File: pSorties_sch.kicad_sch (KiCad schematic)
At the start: 29 parts, among them K1 G6DN-1A-L DC24, K2 G6DN-1A-L DC24, Q1 2N7002, Q2 2N7002, U3 DRV81545PWPR, U4 ISO6420FDR, U5 TLV709A50DBVR

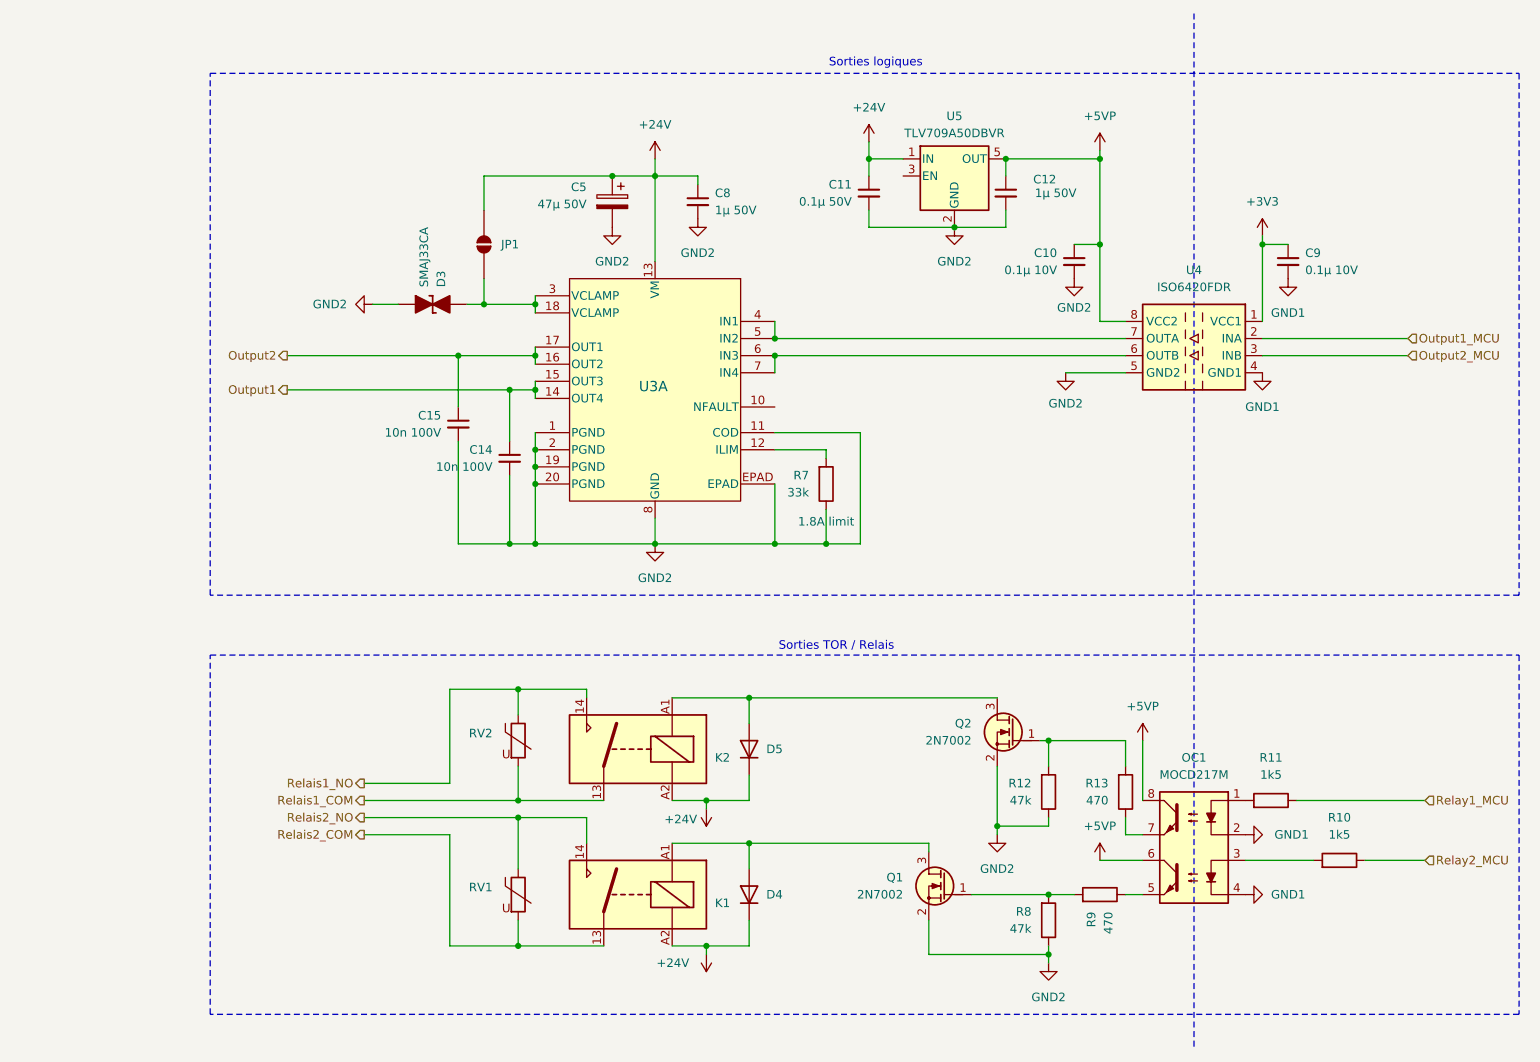
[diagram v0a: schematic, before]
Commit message: avant prod
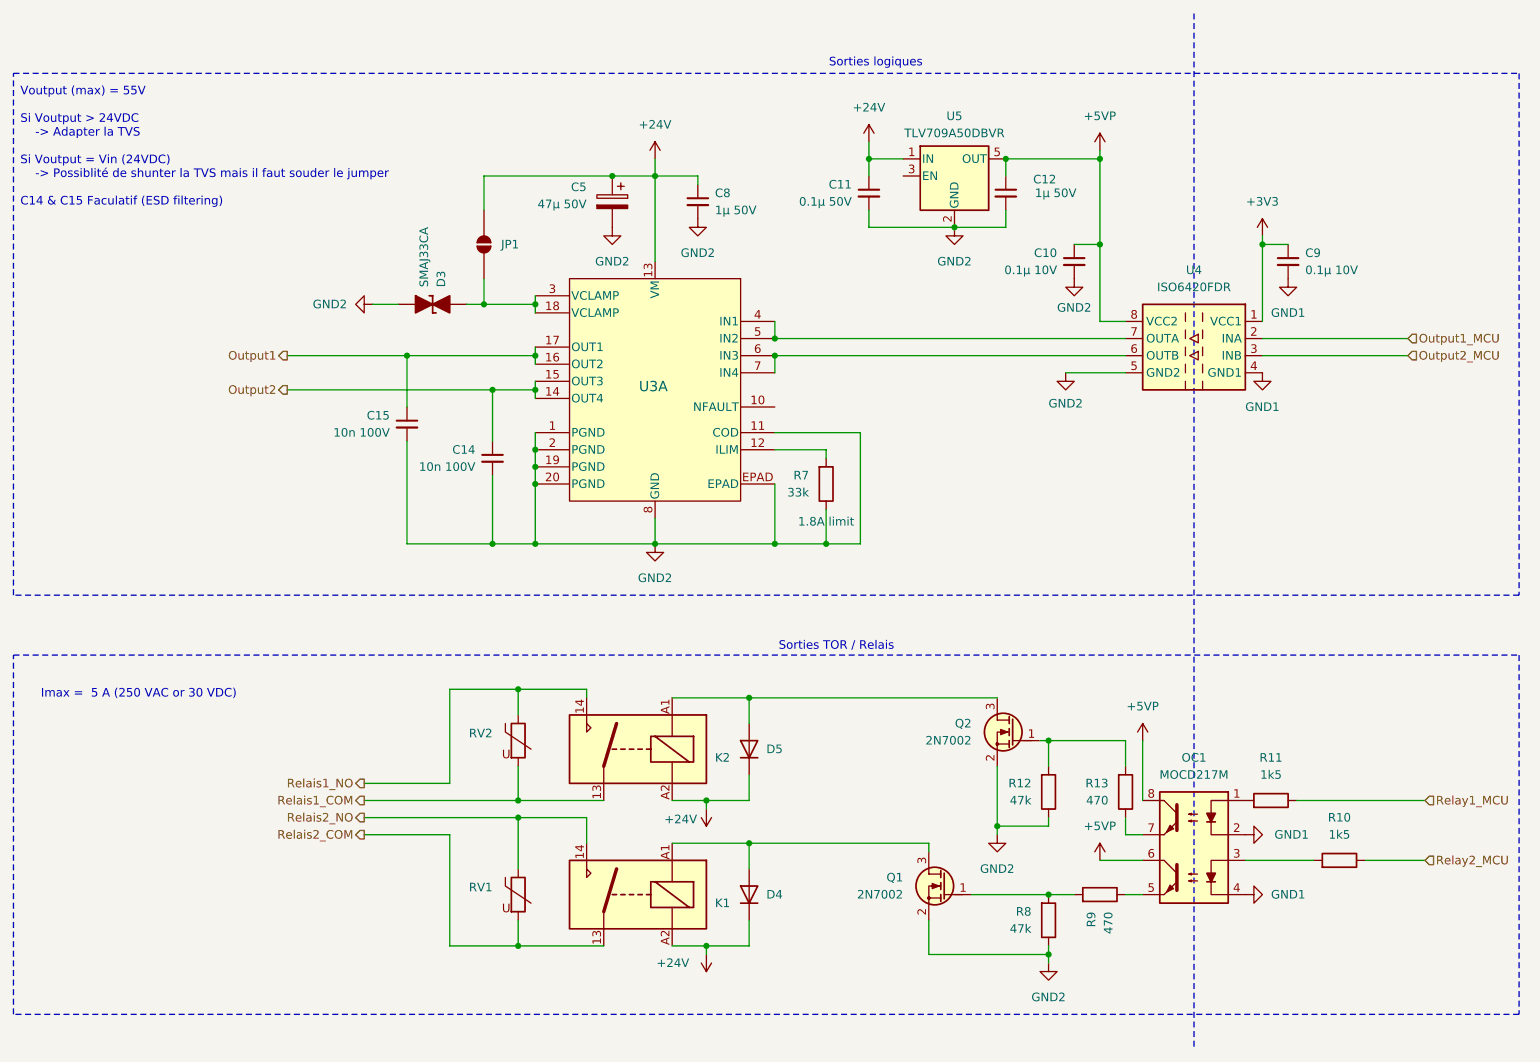
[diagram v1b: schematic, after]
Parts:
- OC1: LCSC Part # (none) -> C258262
- Q1, Q2: LCSC Part # (none) -> C8545
- U3: LCSC Part # (none) -> C53201928
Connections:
- net Output1: now also C15.1, U3.16 (OUT2), U3.17 (OUT1); no longer C14.1, U3.14 (OUT4), U3.15 (OUT3)
- net Output2: now also C14.1, U3.14 (OUT4), U3.15 (OUT3); no longer C15.1, U3.16 (OUT2), U3.17 (OUT1)
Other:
- note added: "Imax = 5 A (250 VAC or 30 VDC)"
- note added: "Voutput (max) = 55V Si Voutput > 24VDC -> Adapter la TVS Si Voutput = Vin (24VDC) -> Possiblité de shunter la TVS mais il faut souder le jumper C14 & C15 Faculatif (ESD filtering)"
- moved on the sheet: C14, C15
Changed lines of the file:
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@@
 	(paper "A4")
 	(rectangle
-		(start 62.23 21.59)
+		(start 33.02 21.59)
 		(end 256.54 99.06)
 		(stroke
@@
 	)
 	(rectangle
-		(start 62.23 107.95)
+		(start 33.02 107.95)
 		(end 256.54 161.29)
 		(stroke
@@
 		)
 	)
+	(text "Voutput (max) = 55V\n\nSi Voutput > 24VDC \n	-> Adapter la TVS\n\nSi Voutput = Vin (24VDC)\n	-> Possiblité de shunter la TVS mais il faut souder le jumper\n\nC14 & C15 Faculatif (ESD filtering)"
+		(exclude_from_sim no)
+		(at 34.036 23.622 0)
+		(effects
+			(font
+				(size 1.27 1.27)
+			)
+			(justify left top)
+		)
+	)
+	(text "Imax =  5 A (250 VAC or 30 VDC)"
+		(exclude_from_sim no)
+		(at 37.084 113.03 0)
+		(effects
+			(font
+				(size 1.27 1.27)
+			)
+			(justify left top)
+		)
+	)
 	(text "Sorties logiques"
 		(exclude_from_sim no)
@@
 	)
 	(junction
-		(at 106.68 68.58)
-		(diameter 0)
-		(color 0 0 0 0)
-	)
-	(junction
 		(at 146.05 63.5)
 		(diameter 0)
@@
 	)
 	(junction
-		(at 99.06 63.5)
+		(at 186.69 152.4)
 		(diameter 0)
 		(color 0 0 0 0)
 	)
 	(junction
-		(at 106.68 91.44)
+		(at 142.24 135.89)
 		(diameter 0)
 		(color 0 0 0 0)
 	)
 	(junction
-		(at 186.69 152.4)
+		(at 104.14 68.58)
 		(diameter 0)
 		(color 0 0 0 0)
 	)
 	(junction
-		(at 142.24 135.89)
+		(at 135.89 151.13)
 		(diameter 0)
 		(color 0 0 0 0)
 	)
 	(junction
-		(at 135.89 151.13)
+		(at 142.24 114.3)
 		(diameter 0)
 		(color 0 0 0 0)
 	)
 	(junction
-		(at 142.24 114.3)
+		(at 146.05 91.44)
 		(diameter 0)
 		(color 0 0 0 0)
 	)
 	(junction
-		(at 146.05 91.44)
+		(at 91.44 63.5)
 		(diameter 0)
 		(color 0 0 0 0)
@@
 	)
 	(junction
+		(at 104.14 91.44)
+		(diameter 0)
+		(color 0 0 0 0)
+	)
+	(junction
 		(at 153.67 91.44)
 		(diameter 0)
@@
 	(wire
 		(pts
-			(xy 106.68 91.44) (xy 110.49 91.44)
-		)
-		(stroke
-			(width 0)
-			(type default)
-		)
-	)
-	(wire
-		(pts
 			(xy 198.12 66.04) (xy 189.23 66.04)
 		)
@@
 	(wire
 		(pts
-			(xy 106.68 81.28) (xy 106.68 91.44)
+			(xy 104.14 81.28) (xy 104.14 91.44)
 		)
 		(stroke
@@
 	(wire
 		(pts
-			(xy 73.66 63.5) (xy 99.06 63.5)
+			(xy 73.66 63.5) (xy 91.44 63.5)
 		)
 		(stroke
@@
 	(wire
 		(pts
+			(xy 104.14 68.58) (xy 110.49 68.58)
+		)
+		(stroke
+			(width 0)
+			(type default)
+		)
+	)
+	(wire
+		(pts
 			(xy 142.24 125.73) (xy 142.24 129.54)
 		)
@@
 	(wire
 		(pts
-			(xy 99.06 63.5) (xy 99.06 71.12)
+			(xy 91.44 63.5) (xy 91.44 71.12)
 		)
 		(stroke
@@
 	(wire
 		(pts
-			(xy 106.68 68.58) (xy 106.68 76.2)
+			(xy 104.14 68.58) (xy 104.14 76.2)
 		)
 		(stroke
@@
 	(wire
 		(pts
-			(xy 99.06 91.44) (xy 106.68 91.44)
+			(xy 91.44 91.44) (xy 104.14 91.44)
 		)
 		(stroke
@@
 	(wire
 		(pts
-			(xy 73.66 68.58) (xy 106.68 68.58)
+			(xy 73.66 68.58) (xy 104.14 68.58)
 		)
 		(stroke
@@
 	(wire
 		(pts
+			(xy 91.44 63.5) (xy 110.49 63.5)
+		)
+		(stroke
+			(width 0)
+			(type default)
+		)
+	)
+	(wire
+		(pts
 			(xy 85.09 132.08) (xy 107.95 132.08)
 		)
@@
 	(wire
 		(pts
+			(xy 104.14 91.44) (xy 110.49 91.44)
+		)
+		(stroke
+			(width 0)
+			(type default)
+		)
+	)
+	(wire
+		(pts
 			(xy 130.81 114.3) (xy 142.24 114.3)
 		)
@@
 	(wire
 		(pts
-			(xy 99.06 76.2) (xy 99.06 91.44)
+			(xy 91.44 76.2) (xy 91.44 91.44)
 		)
 		(stroke
@@
 	(wire
 		(pts
-			(xy 106.68 68.58) (xy 110.49 68.58)
-		)
-		(stroke
-			(width 0)
-			(type default)
-		)
-	)
-	(wire
-		(pts
 			(xy 218.44 45.72) (xy 218.44 46.99)
 		)
@@
 	(wire
 		(pts
-			(xy 99.06 63.5) (xy 110.49 63.5)
-		)
-		(stroke
-			(width 0)
-			(type default)
-		)
-	)
-	(wire
-		(pts
 			(xy 194.31 46.99) (xy 194.31 58.42)
 		)
@@
 		)
 	)
-	(hierarchical_label "Output1"
+	(hierarchical_label "Output2"
 		(shape output)
 		(at 73.66 68.58 180)
@@
 		)
 	)
-	(hierarchical_label "Output2"
+	(hierarchical_label "Output1"
 		(shape output)
 		(at 73.66 63.5 180)
@@
 			)
 		)
+		(property "LCSC Part #" "C8545"
+			(at 171.45 142.24 0)
+			(hide yes)
+			(show_name no)
+			(do_not_autoplace no)
+			(effects
+				(font
+					(size 1.27 1.27)
+				)
+			)
+		)
 		(pin "3"
 		)
@@
 			)
 		)
+		(property "LCSC Part #" "C258262"
+			(at 208.28 132.08 0)
+			(hide yes)
+			(show_name no)
+			(do_not_autoplace no)
+			(effects
+				(font
+					(size 1.27 1.27)
+				)
+			)
+		)
 		(pin "1"
 		)
@@
 	(symbol
 		(lib_id "Device:C_Small")
-		(at 99.06 73.66 0)
+		(at 91.44 73.66 0)
 		(mirror y)
 		(unit 1)
@@
 		(dnp no)
 		(property "Reference" "C15"
-			(at 96.52 72.3962 0)
+			(at 88.9 72.3962 0)
 			(show_name no)
 			(do_not_autoplace no)
@@
 		)
 		(property "Value" "10n 100V"
-			(at 96.52 74.9362 0)
+			(at 88.9 74.9362 0)
 			(show_name no)
 			(do_not_autoplace no)
@@
 		)
 		(property "Footprint" "Capacitor_SMD:C_0603_1608Metric_Pad1.08x0.95mm_HandSolder"
-			(at 99.06 73.66 0)
+			(at 91.44 73.66 0)
 			(hide yes)
 			(show_name no)
@@
 		)
 		(property "Datasheet" "GCM188R71H104KA57D"
-			(at 99.06 73.66 0)
+			(at 91.44 73.66 0)
 			(hide yes)
 			(show_name no)
@@
 		)
 		(property "Description" "Unpolarized capacitor, small symbol"
-			(at 99.06 73.66 0)
+			(at 91.44 73.66 0)
 			(hide yes)
 			(show_name no)
@@
 		)
 		(property "LCSC Part #" "C57112"
-			(at 99.06 73.66 0)
+			(at 91.44 73.66 0)
 			(hide yes)
 			(show_name no)
@@
 		)
 		(property "px_1" "0.086"
-			(at 99.06 73.66 0)
+			(at 91.44 73.66 0)
 			(hide yes)
 			(show_name no)
@@
 		)
 		(property "px_10" "0.02"
-			(at 99.06 73.66 0)
+			(at 91.44 73.66 0)
 			(hide yes)
 			(show_name no)
@@
 		)
 		(property "MPN" "GRM188R72A103MA01J"
-			(at 99.06 73.66 0)
+			(at 91.44 73.66 0)
 			(hide yes)
 			(show_name no)
@@
 			)
 		)
-		(property "Datasheet" ""
+		(property "Datasheet" "https://omronfs.omron.com/en_US/ecb/products/pdf/en-g6dn.pdf"
 			(at 125.73 121.92 0)
 			(hide yes)
@@
 			)
 		)
+		(property "LCSC Part #" "C53201928"
+			(at 128.27 68.58 0)
+			(hide yes)
+			(show_name no)
+			(do_not_autoplace no)
+			(effects
+				(font
+					(size 1.27 1.27)
+				)
+			)
+		)
 		(pin "17"
 		)
@@
 	(symbol
 		(lib_id "Device:C_Small")
-		(at 106.68 78.74 0)
+		(at 104.14 78.74 0)
 		(mirror y)
 		(unit 1)
@@
 		(dnp no)
 		(property "Reference" "C14"
-			(at 104.14 77.4762 0)
+			(at 101.6 77.4762 0)
 			(show_name no)
 			(do_not_autoplace no)
@@
 		)
 		(property "Value" "10n 100V"
-			(at 104.14 80.0162 0)
+			(at 101.6 80.0162 0)
 			(show_name no)
 			(do_not_autoplace no)
@@
 		)
 		(property "Footprint" "Capacitor_SMD:C_0603_1608Metric_Pad1.08x0.95mm_HandSolder"
-			(at 106.68 78.74 0)
+			(at 104.14 78.74 0)
 			(hide yes)
 			(show_name no)
@@
 		)
 		(property "Datasheet" "GCM188R71H104KA57D"
-			(at 106.68 78.74 0)
+			(at 104.14 78.74 0)
 			(hide yes)
 			(show_name no)
@@
 		)
 		(property "Description" "Unpolarized capacitor, small symbol"
-			(at 106.68 78.74 0)
+			(at 104.14 78.74 0)
 			(hide yes)
 			(show_name no)
@@
 		)
 		(property "LCSC Part #" "C57112"
-			(at 106.68 78.74 0)
+			(at 104.14 78.74 0)
 			(hide yes)
 			(show_name no)
@@
 		)
 		(property "px_1" "0.086"
-			(at 106.68 78.74 0)
+			(at 104.14 78.74 0)
 			(hide yes)
 			(show_name no)
@@
 		)
 		(property "px_10" "0.02"
-			(at 106.68 78.74 0)
+			(at 104.14 78.74 0)
 			(hide yes)
 			(show_name no)
@@
 		)
 		(property "MPN" "GRM188R72A103MA01J"
-			(at 106.68 78.74 0)
+			(at 104.14 78.74 0)
 			(hide yes)
 			(show_name no)
@@
 			)
 		)
+		(property "LCSC Part #" "C8545"
+			(at 181.61 119.38 0)
+			(hide yes)
+			(show_name no)
+			(do_not_autoplace no)
+			(effects
+				(font
+					(size 1.27 1.27)
+				)
+			)
+		)
 		(pin "3"
 		)
@@
 			)
 		)
-		(property "Datasheet" ""
+		(property "Datasheet" "https://omronfs.omron.com/en_US/ecb/products/pdf/en-g6dn.pdf"
 			(at 125.73 143.51 0)
 			(hide yes)
